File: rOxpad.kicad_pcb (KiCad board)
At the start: 2 copper layers, 67.5 x 65.1 mm, 25 parts, among them SW1 SW_Push, U1 ATmega16U2-A, U2 PRTR5V0U2X, Y1 16MHz

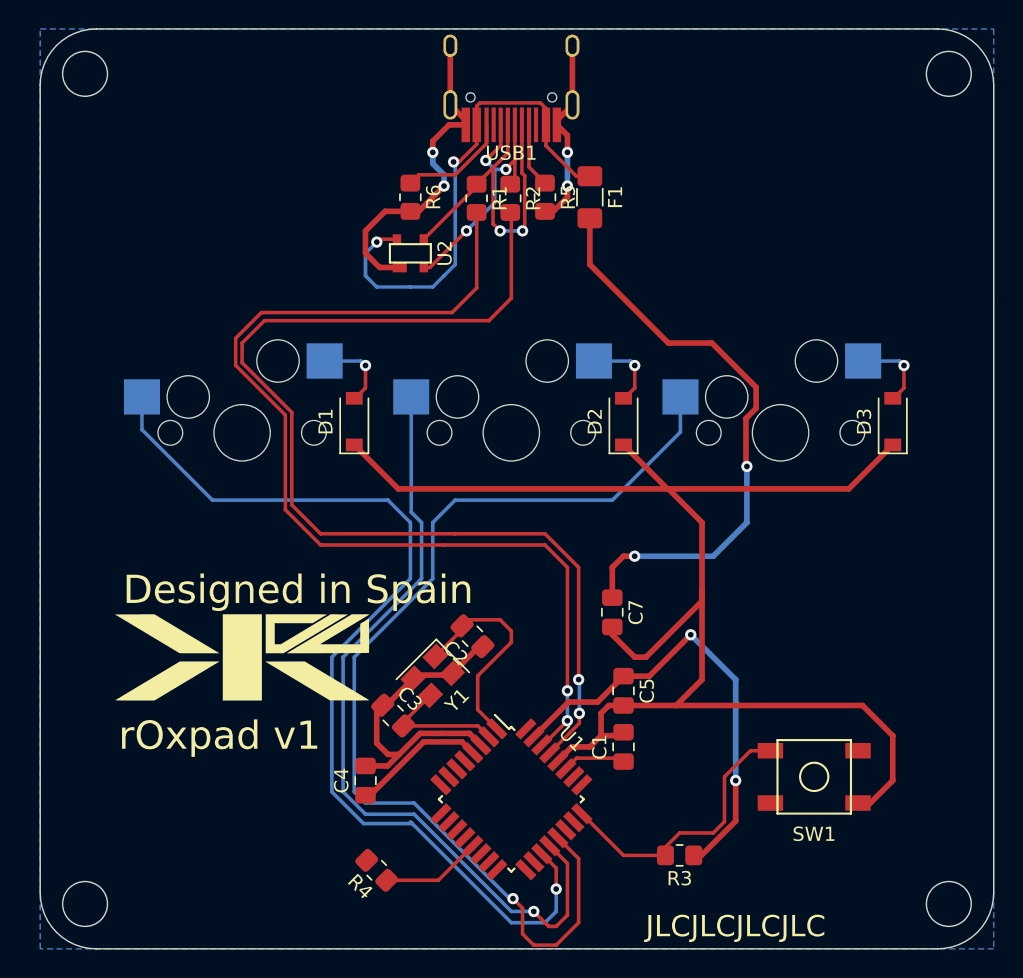
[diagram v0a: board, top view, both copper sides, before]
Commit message: Fix sizing
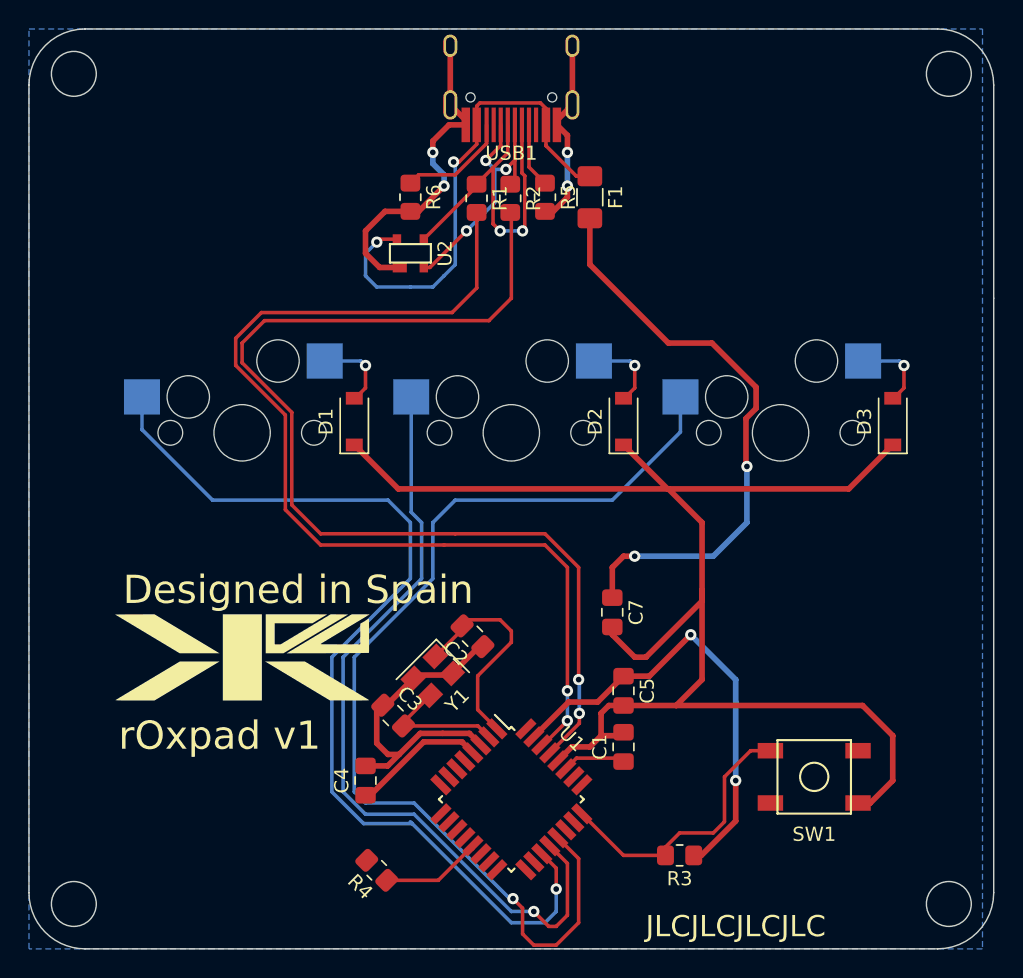
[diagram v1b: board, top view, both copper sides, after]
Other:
- board size 67.5 x 65.1 mm -> 68.3 x 65.1 mm
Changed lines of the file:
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@@
   (gr_arc (start 141.2875 121.44375) (mid 140.12508 124.25008) (end 137.31875 125.4125) (layer "Edge.Cuts") (width 0.1))
   (gr_circle (center 138.1125 122.2375) (end 139.7 122.2375) (layer "Edge.Cuts") (width 0.1) (fill none))
-  (gr_arc (start 77.7875 125.4125) (mid 74.98117 124.25008) (end 73.81875 121.44375) (layer "Edge.Cuts") (width 0.1))
-  (gr_line (start 77.7875 125.4125) (end 137.31875 125.4125) (layer "Edge.Cuts") (width 0.1))
+  (gr_arc (start 76.99375 125.4125) (mid 74.187402 124.250083) (end 73.025 121.44375) (layer "Edge.Cuts") (width 0.1))
+  (gr_line (start 76.99375 125.4125) (end 137.31875 125.4125) (layer "Edge.Cuts") (width 0.1))
   (gr_arc (start 137.31875 60.325) (mid 140.12508 61.48742) (end 141.2875 64.29375) (layer "Edge.Cuts") (width 0.1))
-  (gr_circle (center 76.99375 63.5) (end 76.99375 61.9125) (layer "Edge.Cuts") (width 0.1) (fill none))
-  (gr_line (start 137.31875 60.325) (end 77.7875 60.325) (layer "Edge.Cuts") (width 0.1))
+  (gr_circle (center 76.2 63.5) (end 76.2 61.9125) (layer "Edge.Cuts") (width 0.1) (fill none))
+  (gr_line (start 137.31875 60.325) (end 76.99375 60.325) (layer "Edge.Cuts") (width 0.1))
   (gr_line (start 141.2875 121.44375) (end 141.2875 79.375) (layer "Edge.Cuts") (width 0.1))
-  (gr_line (start 73.81875 64.29375) (end 73.81875 121.44375) (layer "Edge.Cuts") (width 0.1))
-  (gr_circle (center 76.99375 122.2375) (end 76.99375 120.65) (layer "Edge.Cuts") (width 0.1) (fill none))
+  (gr_line (start 73.025 64.29375) (end 73.025 121.44375) (layer "Edge.Cuts") (width 0.1))
+  (gr_circle (center 76.2 122.2375) (end 76.2 120.65) (layer "Edge.Cuts") (width 0.1) (fill none))
   (gr_line (start 141.2875 79.375) (end 141.2875 64.29375) (layer "Edge.Cuts") (width 0.1))
-  (gr_arc (start 73.81875 64.29375) (mid 74.98117 61.48742) (end 77.7875 60.325) (layer "Edge.Cuts") (width 0.1))
+  (gr_arc (start 73.025 64.29375) (mid 74.18742 61.48742) (end 76.99375 60.325) (layer "Edge.Cuts") (width 0.1))
   (gr_text "Designed in Spain" (at 92.075 100.0125) (layer "F.SilkS")
     (effects (font (size 2 2) (thickness 0.15)))
@@
     (polygon
       (pts
-        (xy 141.2875 125.4125)
-        (xy 73.81875 125.4125)
-        (xy 73.81875 60.325)
-        (xy 141.2875 60.325)
+        (xy 140.49375 125.4125)
+        (xy 73.025 125.4125)
+        (xy 73.025 60.325)
+        (xy 140.49375 60.325)
       )
     )
